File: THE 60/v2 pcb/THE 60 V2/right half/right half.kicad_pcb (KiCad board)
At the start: 2 copper layers, 141.7 x 107.7 mm, 70 parts, among them J1 Conn_01x02_Socket, SW1 Switch, SW2 Switch, U2 Nice_Nano_V2, U3 TRRS

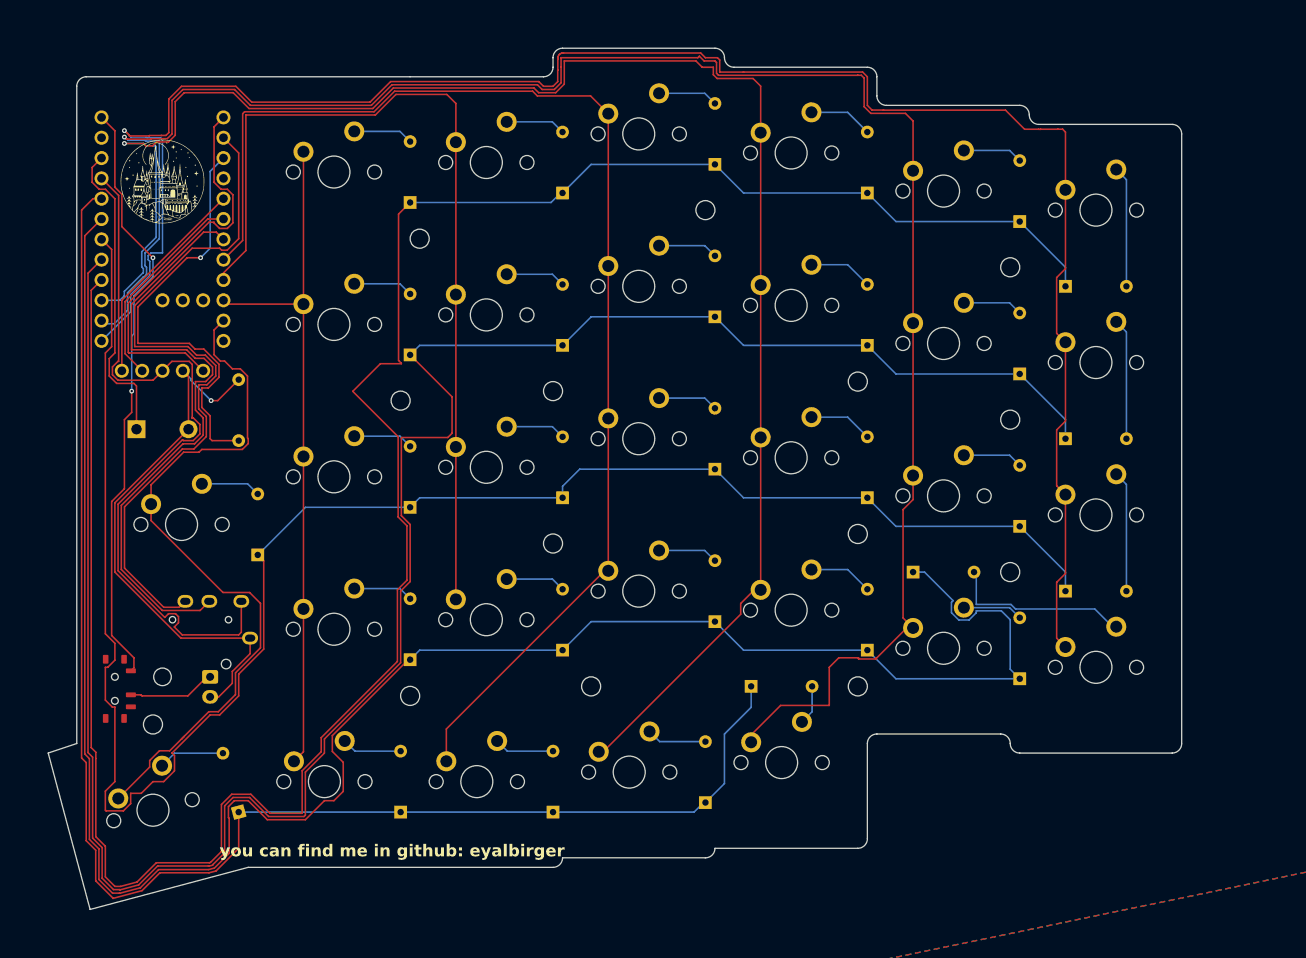
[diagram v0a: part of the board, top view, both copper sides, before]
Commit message: z
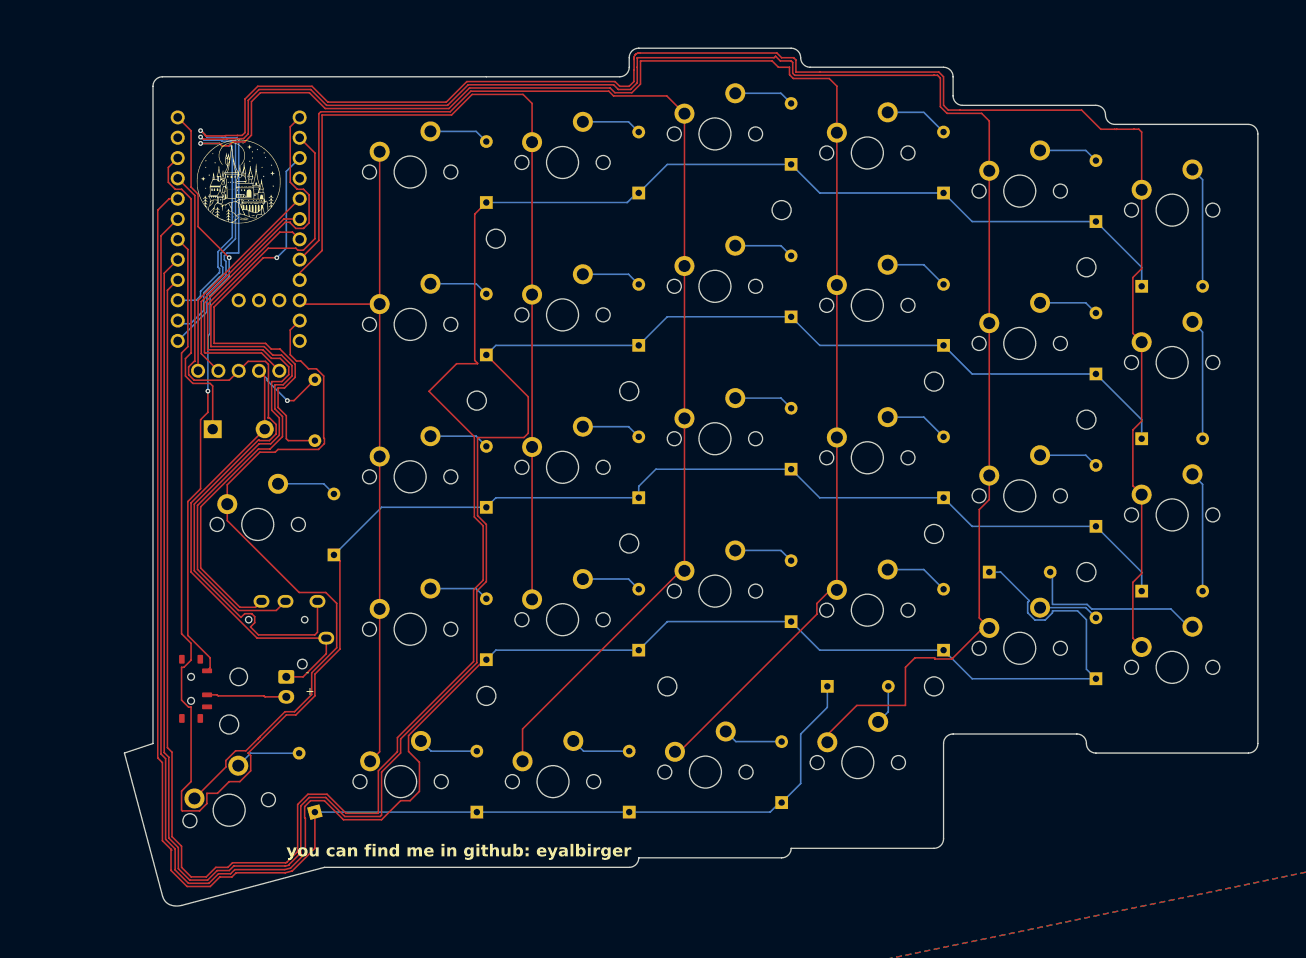
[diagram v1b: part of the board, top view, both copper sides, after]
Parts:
- moved D1 9.53 mm to (167.5, 76.1)
- moved D11 9.53 mm to (243.7, 97.5)
- moved D12 9.53 mm to (249.4, 105.6)
- moved D13 9.53 mm to (167.5, 114.2)
- moved D14 9.53 mm to (186.6, 113.0)
- moved D15 9.53 mm to (205.6, 109.4)
- moved D17 9.53 mm to (243.7, 116.6)
- moved D18 9.53 mm to (249.4, 124.7)
- moved D19 9.53 mm to (167.5, 133.2)
- moved D2 9.53 mm to (186.6, 74.9)
- moved D20 9.53 mm to (186.6, 132.0)
- moved D21 9.53 mm to (205.6, 128.5)
- moved D23 9.53 mm to (243.7, 135.6)
- moved D24 9.53 mm to (230.4, 122.3)
- moved D25 9.53 mm to (148.5, 120.1)
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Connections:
- J1 pad 1: + -> gnd
- J1 pad 2: gnd -> +
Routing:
- net row 3: track 253.0 -> 251.5 mm
- net row 1: track 277.1 -> 275.5 mm
- net row 0: track 291.0 -> 289.4 mm
- net row 4: track 189.8 -> 188.3 mm
- net gnd: track 69.6 -> 68.1 mm
- net +: track 10.9 -> 10.0 mm
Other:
- board size 141.7 x 107.7 mm -> 141.7 x 107.2 mm
- board text added: "+"
- board text added: "-"
